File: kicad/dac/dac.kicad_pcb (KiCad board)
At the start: 4 copper layers, 69.8 x 45 mm, 52 parts, among them U1 ES9039Q2M, U2 OPA1612AxD, U3 OPA1612AxD, U4 LT3046ATC+

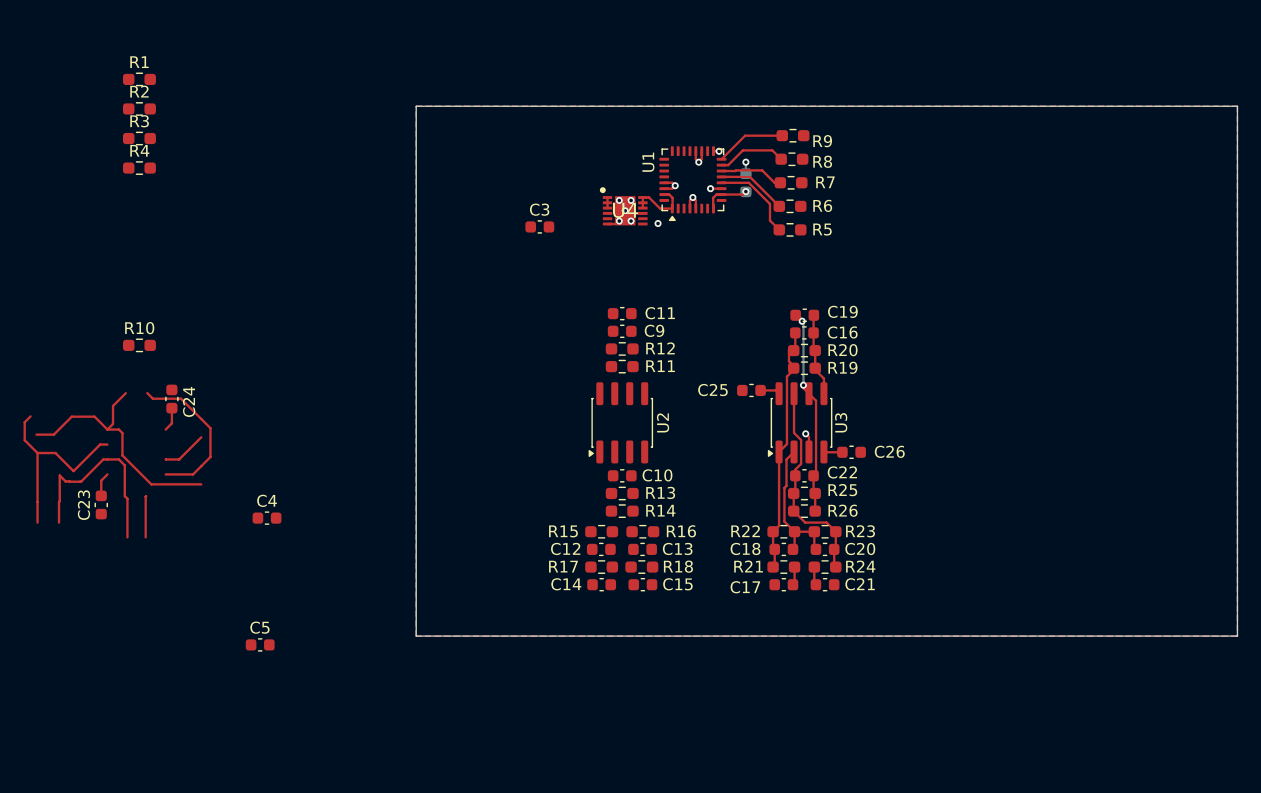
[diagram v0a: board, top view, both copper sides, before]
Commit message: WIP
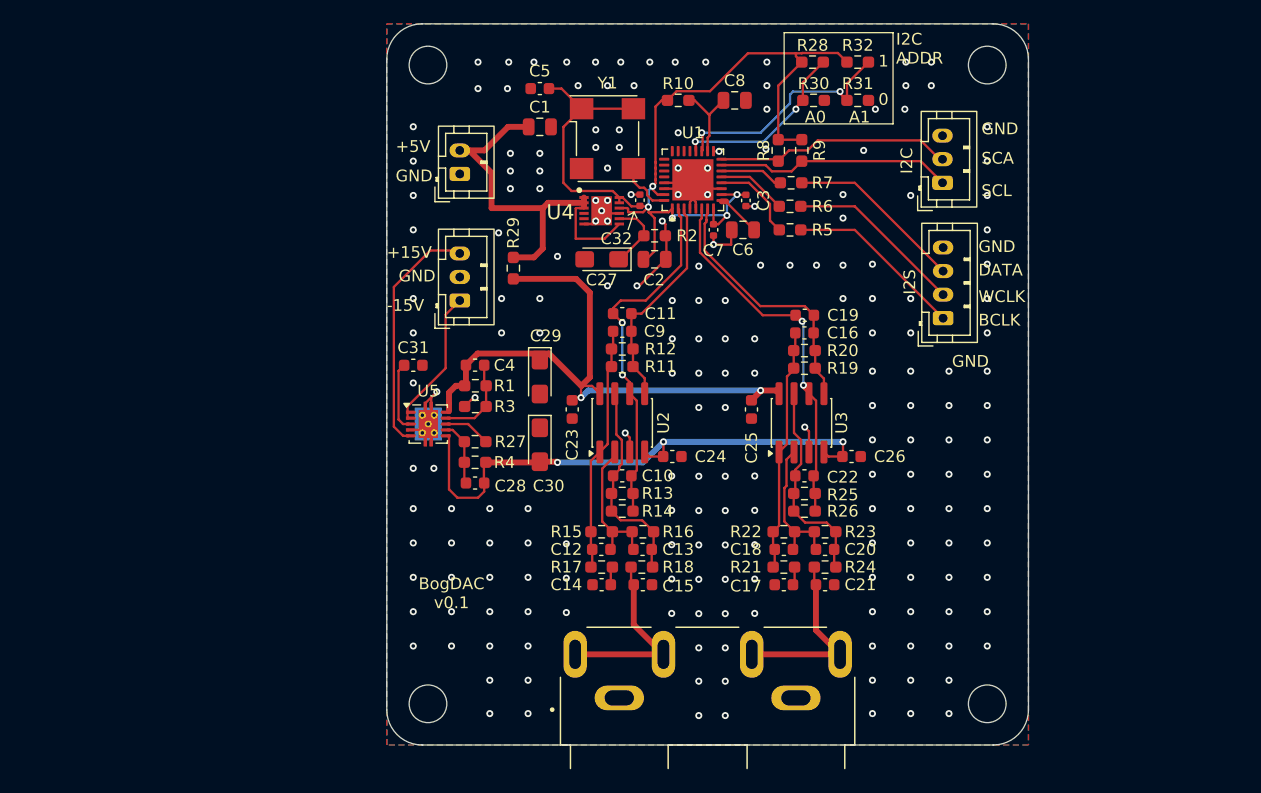
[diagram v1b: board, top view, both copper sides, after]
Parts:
- added C1: 10u, Capacitor_SMD:C_0805_2012Metric, F.Cu at (115.5, 83.5)
- added C2: 10u, Capacitor_SMD:C_0805_2012Metric, F.Cu at (125.2, 94.8)
- added C27: 22u, Capacitor_Tantalum_SMD:CP_EIA-3216-10_Kemet-I_HandSolder, F.Cu at (120.8, 94.8)
- added C28: 10n, Capacitor_SMD:C_0603_1608Metric, F.Cu at (110.0, 113.8)
- added C29: 22u, Capacitor_Tantalum_SMD:CP_EIA-3216-10_Kemet-I_HandSolder, F.Cu at (115.5, 104.8)
- added C30: 22u, Capacitor_Tantalum_SMD:CP_EIA-3216-10_Kemet-I_HandSolder, F.Cu at (115.5, 110.5)
- added C31: 10n, Capacitor_SMD:C_0603_1608Metric, F.Cu at (104.8, 103.8)
- added C32: 100n, Capacitor_SMD:C_0402_1005Metric, F.Cu at (124.0, 89.7)
- added C6: 10u, Capacitor_SMD:C_0805_2012Metric, F.Cu at (132.8, 92.2)
- added C8: 10u, Capacitor_SMD:C_0805_2012Metric, F.Cu at (132.1, 81.2)
- added H1: MountingHole, MountingHole:MountingHole_3.2mm_M3, F.Cu at (106.0, 78.2)
- added H2: MountingHole, MountingHole:MountingHole_3.2mm_M3, F.Cu at (153.5, 78.2)
- added H3: MountingHole, MountingHole:MountingHole_3.2mm_M3, F.Cu at (153.5, 132.5)
- added H4: MountingHole, MountingHole:MountingHole_3.2mm_M3, F.Cu at (106.0, 132.5)
- added J1: I2S, Connector_JST:JST_PH_B3B-PH-K_1x03_P2.00mm_Vertical, F.Cu at (149.7, 88.2)
- added J2: I2S, Connector_JST:JST_PH_B4B-PH-K_1x04_P2.00mm_Vertical, F.Cu at (149.8, 99.8)
- added J3: ANALOG PWR, Connector_JST:JST_PH_B3B-PH-K_1x03_P2.00mm_Vertical, F.Cu at (108.7, 98.2)
- added J4: 5V, Connector_JST:JST_PH_B2B-PH-K_1x02_P2.00mm_Vertical, F.Cu at (108.7, 87.5)
- added J5: AUDIO OUT, Custom:SWITCHCRAFT_PJRAN2X1U01AUX, F.Cu at (129.8, 136.0)
- added R27: 10k, Resistor_SMD:R_0603_1608Metric_Pad0.98x0.95mm_HandSolder, F.Cu at (110.0, 110.2)
- added R28: 0, Resistor_SMD:R_0603_1608Metric_Pad0.98x0.95mm_HandSolder, F.Cu at (138.7, 78.0)
- added R29: 0, Resistor_SMD:R_0603_1608Metric_Pad0.98x0.95mm_HandSolder, F.Cu at (113.2, 95.5)
- added R30: 0, Resistor_SMD:R_0603_1608Metric_Pad0.98x0.95mm_HandSolder, F.Cu at (138.8, 81.2)
- added R31: 0, Resistor_SMD:R_0603_1608Metric_Pad0.98x0.95mm_HandSolder, F.Cu at (142.5, 81.2)
- added R32: 0, Resistor_SMD:R_0603_1608Metric_Pad0.98x0.95mm_HandSolder, F.Cu at (142.5, 78.0)
- added REF**: logo2, Custom:logo2, F.Cu at (151.0, 130.5)
- added REF**: logo2, Custom:logo2, F.Cu at (115.2, 130.5)
- added REF**: logo2, Custom:logo2, F.Cu at (112.0, 130.5)
- added REF**: logo2, Custom:logo2, F.Cu at (144.5, 130.5)
- added REF**: logo2, Custom:logo2, F.Cu at (105.5, 130.5)
- added REF**: logo2, Custom:logo2, F.Cu at (154.2, 130.5)
- added REF**: logo2, Custom:logo2, F.Cu at (147.8, 130.5)
- added REF**: logo2, Custom:logo2, F.Cu at (108.8, 130.5)
- added U5: TPS7A39, Package_SON:Texas_S-PVSON-N10_ThermalVias, F.Cu at (106.0, 108.7)
- added Y1: CE3391-49.152, Oscillator:Oscillator_SMD_Diodes_FN-4Pin_7.0x5.0mm, F.Cu at (121.2, 84.5)
- C3: footprint Capacitor_SMD:C_0603_1608Metric -> Capacitor_SMD:C_0402_1005Metric
- C4: value 100n -> 10n
- C7: footprint Capacitor_SMD:C_0603_1608Metric -> Capacitor_SMD:C_0402_1005Metric; moved to F.Cu
- R1: value 200k -> 90.9k
- R10: value 100k -> 47k
- R3: value 453k -> 10k
- R4: value 49.9k -> 100k
- R8, R9: value 50 -> 4.7k
- U1: footprint Package_DFN_QFN:UQFN-32_5x5mm_P0.5mm -> Package_DFN_QFN:UFQFPN-32-1EP_5x5mm_P0.5mm_EP3.5x3.5mm
- moved C5 52.9 mm to (115.5, 80.2), turned to 180 degrees
- moved R10 50.3 mm to (127.2, 81.2)
- moved R2 45.1 mm to (125.2, 92.8)
- moved C24 42.8 mm to (126.8, 111.5), turned to 0 degrees
- moved C23 40.8 mm to (118.2, 107.5)
- moved R1 38.6 mm to (110.0, 105.5)
- moved R4 37.9 mm to (110.0, 112.0)
- moved R3 36.5 mm to (110.0, 107.2)
- moved C4 21.9 mm to (110.0, 103.7)
- moved C3 17.6 mm to (133.0, 89.8), turned to -90 degrees
- moved C7 4.85 mm to (130.2, 92.2), turned to -90 degrees
- moved U4 2.00 mm to (120.8, 90.6)
- moved C25 1.61 mm to (133.5, 107.5), turned to 90 degrees
- moved R9 1.46 mm to (137.8, 85.5), turned to -90 degrees
- moved R8 1.38 mm to (135.8, 85.5), turned to -90 degrees
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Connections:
- C4 pad 1: GND -> +12V
- C4 pad 2: +3.3V -> Net-(U5-FBP)
- R1 pad 1: +5V -> +12V
- R1 pad 2: Net-(U4-PG) -> Net-(U5-FBP)
- R3 pad 1: +3.3V -> GND
- R3 pad 2: Net-(U4-PGFB) -> Net-(U5-FBP)
- R4 pad 1: Net-(U4-PGFB) -> Net-(U5-FBN)
- R4 pad 2: GND -> -12V
- R8 pad 1: Net-(U1-SCL) -> +3.3V
- R8 pad 2: /SCL -> /SCA
- R9 pad 1: Net-(U1-SCA) -> +3.3V
- R9 pad 2: /SCA -> /SCL
- U1 pad 15: Net-(U1-SCL) -> /SCL
- U1 pad 16: Net-(U1-SCA) -> /SCA
- U1 pad 19: GND -> Net-(U1-ADDR1)
- U1 pad 20: GND -> Net-(U1-ADDR0)
- U4 pad 7: unconnected-(U4-PGFB-Pad7) -> +5V
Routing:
- net +3.3V: track 9.45 -> 85.0 mm, vias 1 -> 5
- net +12V: track 3.72 -> 53.5 mm, vias 0 -> 2
- net -12V: track 3.62 -> 47.7 mm, vias 0 -> 3
- net +5V: track 0.90 -> 35.8 mm
- net /-15V: track 0.00 -> 20.3 mm
- net Net-(U1-ADDR1): track 0.00 -> 20.3 mm, vias 0 -> 2
- net /SCL: track 0.00 -> 20.2 mm
- net /SCA: track 0.00 -> 20.0 mm
- net GND: track 13.2 -> 32.6 mm, vias 13 -> 201
- net Net-(C15-Pad2): track 0.00 -> 16.1 mm
- net Net-(U1-ADDR0): track 0.00 -> 15.5 mm, vias 0 -> 2
- net DAC2: track 6.90 -> 22.1 mm
- net /WCLK: track 0.00 -> 15.2 mm
- net /BCLK: track 0.00 -> 15.2 mm
- net /DATA: track 0.00 -> 15.1 mm
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- added copper zone on In2.Cu, net GND
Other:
- board size 69.8 x 45 mm -> 54.5 x 61.2 mm
- board text added: "+15V"
- board text added: "+5V"
- board text added: "-15V"
- board text added: "0"
- board text added: "1"
- board text added: "A0"
- board text added: "A1"
- board text added: "BCLK"
- board text added: "BogDAC v0.1"
- board text added: "DATA"
- board text added: "GND"
- board text added: "I2C"
- board text added: "I2C ADDR"
- board text added: "I2S"
- board text added: "SCA"
- board text added: "SCL"
- board text added: "WCLK"
